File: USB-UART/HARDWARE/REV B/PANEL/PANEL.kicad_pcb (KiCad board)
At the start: 2 copper layers, 81.8 x 90.9 mm, 393 parts, among them P1 USB_OTG, P2 LEFT, P3 RIGHT, U1 FT230XQ-R, U2 AP1117

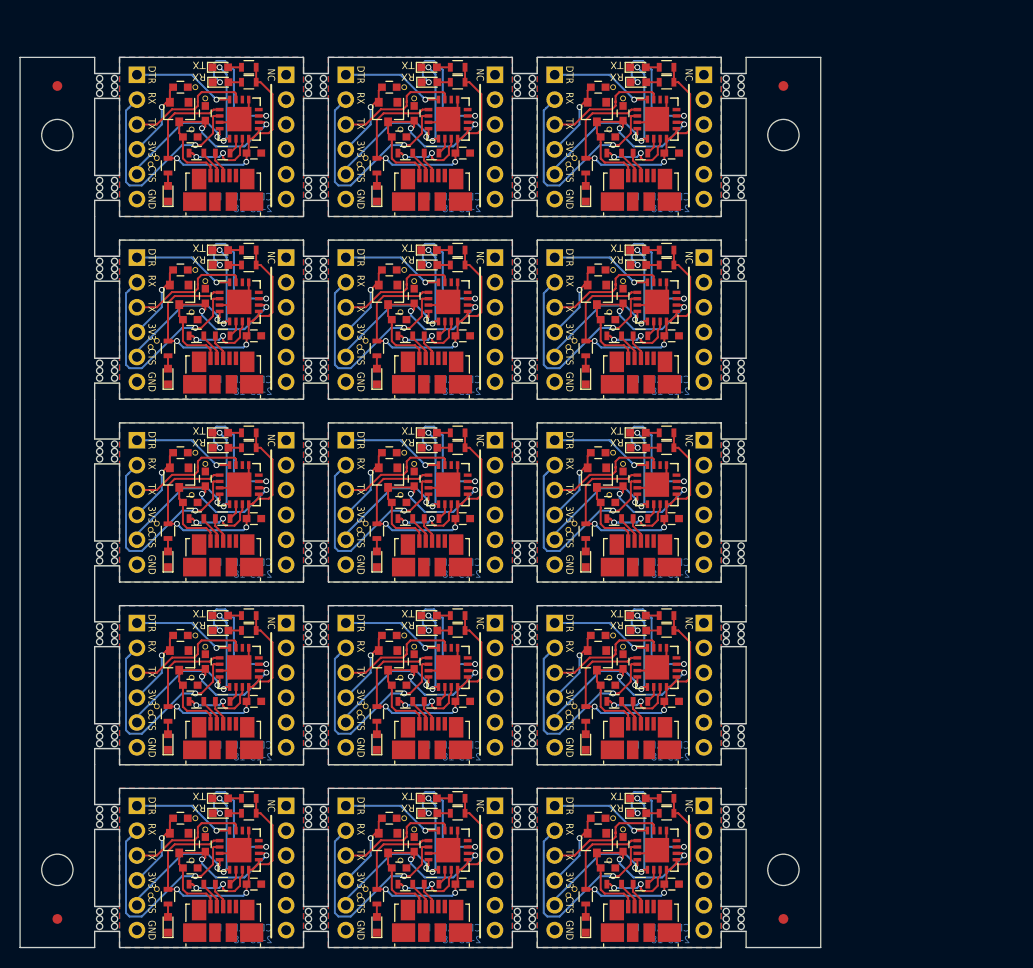
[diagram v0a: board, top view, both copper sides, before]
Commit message: file recovery and updates
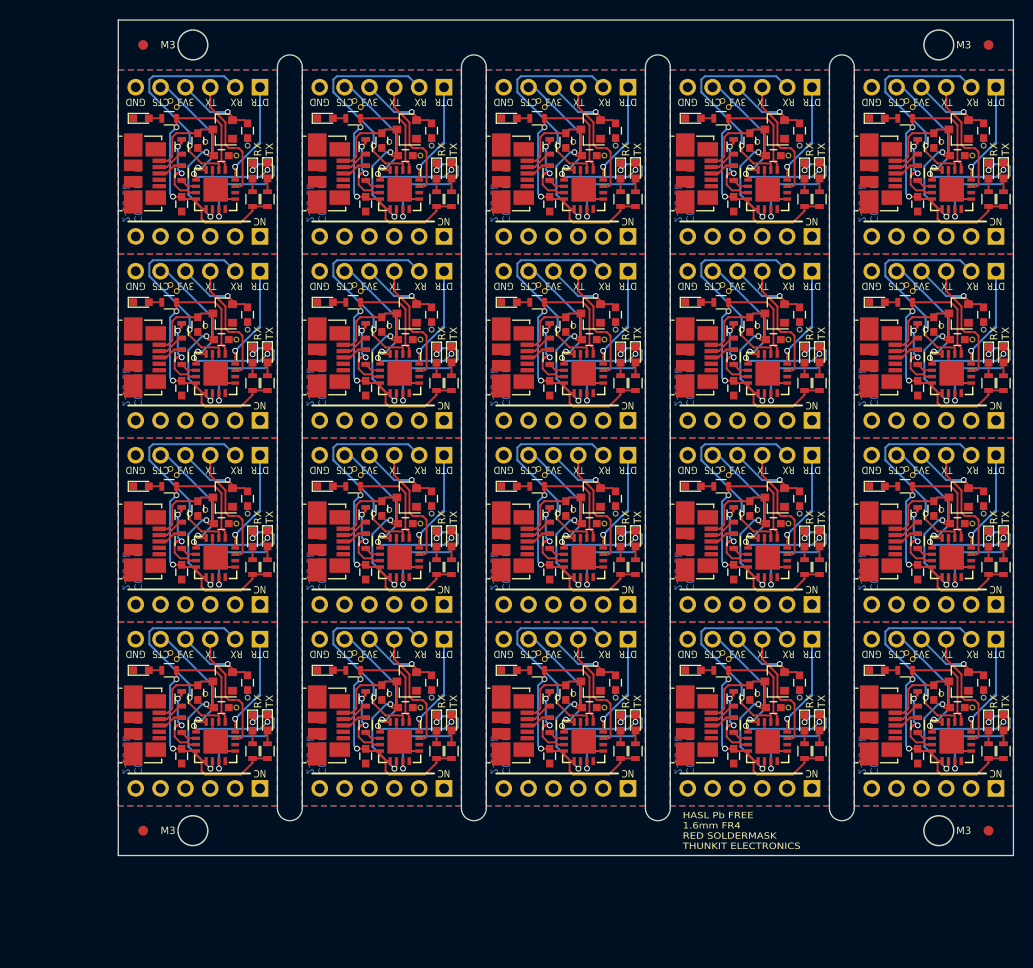
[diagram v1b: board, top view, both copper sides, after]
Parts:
- removed the ? at (164.0, 134.4)
- removed the ? at (121.3, 134.4)
- removed the ? at (125.2, 127.1)
- removed the ? at (126.2, 128.3)
- removed the ? at (124.8, 131.4)
- removed the ? at (146.2, 131.4)
- removed the ? at (146.6, 127.1)
- removed the ? at (125.2, 108.5)
- removed the ? at (124.8, 112.8)
- removed the ? at (121.3, 115.7)
- removed the ? at (120.7, 116.3)
- removed the ? at (163.3, 135.0)
- removed the ? at (126.2, 109.6)
- removed the ? at (164.0, 115.7)
- removed the ? at (163.3, 116.3)
- removed the ? at (167.5, 112.8)
- removed the ? at (167.9, 108.5)
- removed the ? at (168.9, 109.6)
- removed the ? at (146.6, 108.5)
- removed the ? at (142.0, 116.3)
- removed the ? at (142.6, 115.7)
- removed the ? at (146.2, 112.8)
- removed the ? at (167.9, 127.1)
- removed the ? at (147.6, 109.6)
- removed the ? at (168.9, 90.9)
- removed the ? at (167.9, 89.8)
- removed the ? at (167.5, 94.1)
- removed the ? at (164.0, 97.0)
- removed the ? at (163.3, 97.7)
- removed the ? at (147.6, 90.9)
- removed the ? at (146.6, 89.8)
- removed the ? at (146.2, 94.1)
- removed the ? at (124.8, 94.1)
- removed the ? at (167.5, 131.4)
- removed the ? at (120.7, 97.7)
- removed the ? at (121.3, 97.0)
- removed the ? at (126.2, 90.9)
- removed the ? at (125.2, 89.8)
- removed the ? at (142.0, 97.7)
- removed the ? at (142.6, 97.0)
- removed the ? at (167.9, 71.1)
- removed the ? at (168.9, 72.3)
- removed the ? at (164.0, 78.4)
- removed the ? at (163.3, 79.0)
- removed the ? at (142.0, 135.0)
- removed the ? at (167.5, 75.4)
- removed the ? at (147.6, 72.3)
- removed the ? at (124.8, 75.4)
- removed the ? at (125.2, 71.1)
- removed the ? at (126.2, 72.3)
- removed the ? at (142.6, 78.4)
- removed the ? at (146.6, 71.1)
- removed the ? at (146.2, 75.4)
- removed the ? at (121.3, 78.4)
- removed the ? at (120.7, 79.0)
- removed the ? at (142.6, 134.4)
- removed the ? at (142.0, 79.0)
- removed the ? at (167.5, 56.8)
- removed the ? at (163.3, 60.3)
- removed the ? at (164.0, 59.7)
- removed the ? at (168.9, 53.6)
- removed the ? at (167.9, 52.5)
- removed the ? at (146.6, 52.5)
- removed the ? at (142.6, 59.7)
- removed the ? at (142.0, 60.3)
- removed the ? at (146.2, 56.8)
- removed the ? at (147.6, 128.3)
- removed the ? at (147.6, 53.6)
- removed the ? at (168.9, 128.3)
- removed the ? at (120.7, 135.0)
- removed the C1 at (152.5, 135.1)
- removed the C1 at (173.9, 79.1)
- removed the C1 at (131.2, 79.1)
- removed the C1 at (152.5, 79.1)
- removed the C1 at (173.9, 60.5)
- removed the C1 at (152.5, 60.5)
- removed the C1 at (173.9, 135.1)
- removed the C1 at (131.2, 135.1)
- removed the C1 at (131.2, 116.5)
- removed the C1 at (173.9, 116.5)
- removed the C1 at (152.5, 116.5)
- removed the C1 at (173.9, 97.8)
- removed the C1 at (152.5, 97.8)
- removed the C1 at (131.2, 97.8)
- removed the C2 at (147.6, 131.1)
- removed the C2 at (168.9, 75.1)
- removed the C2 at (147.6, 75.1)
- removed the C2 at (126.2, 75.1)
- removed the C2 at (168.9, 56.4)
- removed the C2 at (147.6, 56.4)
- removed the C2 at (168.9, 131.1)
- removed the C2 at (126.2, 131.1)
- removed the C2 at (126.2, 112.4)
- removed the C2 at (168.9, 112.4)
- removed the C2 at (147.6, 112.4)
- removed the C2 at (168.9, 93.7)
- removed the C2 at (147.6, 93.7)
- removed the C2 at (126.2, 93.7)
- removed the C3 at (146.0, 133.5)
- removed the C3 at (167.4, 77.5)
- removed the C3 at (124.7, 77.5)
- removed the C3 at (146.0, 77.5)
- removed the C3 at (167.4, 58.8)
- removed the C3 at (146.0, 58.8)
- removed the C3 at (167.4, 133.5)
- removed the C3 at (124.7, 133.5)
- removed the C3 at (124.7, 114.8)
- removed the C3 at (167.4, 114.8)
- removed the C3 at (146.0, 114.8)
- removed the C3 at (167.4, 96.1)
- removed the C3 at (124.7, 96.1)
- removed the C3 at (146.0, 96.1)
- removed the C4 at (166.4, 128.4)
- removed the C4 at (166.4, 72.4)
- removed the C4 at (123.7, 72.4)
- removed the C4 at (145.0, 72.4)
- removed the C4 at (166.4, 53.7)
- removed the C4 at (145.0, 53.7)
- removed the C4 at (123.7, 128.4)
- removed the C4 at (145.0, 128.4)
- removed the C4 at (123.7, 109.7)
- removed the C4 at (166.4, 109.7)
- removed the C4 at (145.0, 109.7)
- removed the C4 at (166.4, 91.1)
- removed the C4 at (145.0, 91.1)
- removed the C4 at (123.7, 91.1)
- removed the D1 at (165.1, 139.3)
- removed the D1 at (165.1, 83.3)
- removed the D1 at (122.4, 83.3)
- removed the D1 at (143.8, 83.3)
- removed the D1 at (165.1, 64.6)
- removed the D1 at (143.8, 64.6)
- removed the D1 at (143.8, 139.3)
- removed the D1 at (122.4, 139.3)
- removed the D1 at (122.4, 120.6)
- removed the D1 at (165.1, 120.6)
- removed the D1 at (143.8, 120.6)
- removed the D1 at (165.1, 101.9)
- removed the D1 at (122.4, 101.9)
- removed the D1 at (143.8, 101.9)
- removed the D2 at (149.1, 126.4)
- removed the D2 at (170.4, 70.4)
- removed the D2 at (149.1, 70.4)
- removed the D2 at (127.8, 70.4)
- removed the D2 at (170.4, 51.7)
- removed the D2 at (149.1, 51.7)
- removed the D2 at (170.4, 126.4)
- removed the D2 at (127.8, 126.4)
- removed the D2 at (127.8, 107.7)
- removed the D2 at (170.4, 107.7)
- removed the D2 at (149.1, 107.7)
- removed the D2 at (170.4, 89.0)
- removed the D2 at (149.1, 89.0)
- removed the D2 at (127.8, 89.0)
- removed the D3 at (149.1, 127.9)
- removed the D3 at (170.5, 71.9)
- removed the D3 at (149.1, 71.9)
- removed the D3 at (127.8, 71.9)
- removed the D3 at (170.5, 53.2)
- removed the D3 at (149.1, 53.2)
- removed the D3 at (170.5, 127.9)
- removed the D3 at (127.8, 127.9)
- removed the D3 at (127.8, 109.2)
- removed the D3 at (170.5, 109.2)
- removed the D3 at (149.1, 109.2)
- removed the D3 at (170.5, 90.6)
- removed the D3 at (149.1, 90.6)
- removed the D3 at (127.8, 90.6)
- removed the G*** at (144.1, 138.0)
- removed the G*** at (144.1, 82.0)
- removed the G*** at (122.8, 82.0)
- removed the G*** at (165.5, 82.0)
- removed the G*** at (165.5, 63.4)
- removed the G*** at (144.1, 63.4)
- removed the G*** at (122.8, 138.0)
- removed the G*** at (165.5, 138.0)
- removed the G*** at (165.5, 119.4)
- removed the G*** at (144.1, 119.4)
- removed the G*** at (122.8, 119.4)
- removed the G*** at (122.8, 100.7)
- removed the G*** at (144.1, 100.7)
- removed the G*** at (165.5, 100.7)
- removed the P1 at (149.4, 140.1)
- removed the P1 at (170.7, 84.1)
- removed the P1 at (128.1, 84.1)
- removed the P1 at (149.4, 84.1)
- removed the P1 at (170.7, 65.4)
- removed the P1 at (149.4, 65.4)
- removed the P1 at (170.7, 140.1)
- removed the P1 at (128.1, 140.1)
- removed the P1 at (128.1, 121.4)
- removed the P1 at (170.7, 121.4)
- removed the P1 at (149.4, 121.4)
- removed the P1 at (170.7, 102.7)
- removed the P1 at (149.4, 102.7)
- removed the P1 at (128.1, 102.7)
- removed the P2 at (140.6, 127.1)
- removed the P2 at (140.6, 71.1)
- removed the P2 at (119.3, 71.1)
- removed the P2 at (161.9, 71.1)
- removed the P2 at (161.9, 52.5)
- removed the P2 at (140.6, 52.5)
- removed the P2 at (119.3, 127.1)
- removed the P2 at (161.9, 127.1)
- removed the P2 at (161.9, 108.5)
- removed the P2 at (140.6, 108.5)
- removed the P2 at (119.3, 108.5)
- removed the P2 at (140.6, 89.8)
- removed the P2 at (119.3, 89.8)
- removed the P2 at (161.9, 89.8)
- removed the P3 at (134.5, 127.1)
- removed the P3 at (134.5, 71.1)
- removed the P3 at (155.8, 71.1)
- removed the P3 at (177.2, 71.1)
- removed the P3 at (177.2, 52.5)
- removed the P3 at (155.8, 52.5)
- removed the P3 at (155.8, 127.1)
- removed the P3 at (177.2, 127.1)
- removed the P3 at (155.8, 108.5)
- removed the P3 at (177.2, 108.5)
- removed the P3 at (134.5, 108.5)
- removed the P3 at (134.5, 89.8)
- removed the P3 at (155.8, 89.8)
- removed the P3 at (177.2, 89.8)
- removed the R1 at (146.7, 135.1)
- removed the R1 at (168.0, 79.1)
- removed the R1 at (125.3, 79.1)
- removed the R1 at (146.7, 79.1)
- removed the R1 at (168.0, 60.5)
- removed the R1 at (146.7, 60.5)
- removed the R1 at (168.0, 135.1)
- removed the R1 at (125.3, 135.1)
- removed the R1 at (125.3, 116.5)
- removed the R1 at (168.0, 116.5)
- removed the R1 at (146.7, 116.5)
- removed the R1 at (168.0, 97.8)
- removed the R1 at (146.7, 97.8)
- removed the R1 at (125.3, 97.8)
- removed the R2 at (149.4, 135.1)
- removed the R2 at (170.7, 79.1)
- removed the R2 at (128.0, 79.1)
- removed the R2 at (149.4, 79.1)
- removed the R2 at (170.7, 60.5)
- removed the R2 at (149.4, 60.5)
- removed the R2 at (170.7, 135.1)
- removed the R2 at (128.0, 135.1)
- removed the R2 at (128.0, 116.5)
- removed the R2 at (170.7, 116.5)
- removed the R2 at (149.4, 116.5)
- removed the R2 at (170.7, 97.8)
- removed the R2 at (149.4, 97.8)
- removed the R2 at (128.0, 97.8)
- removed the R3 at (165.1, 136.4)
- removed the R3 at (165.1, 80.4)
- removed the R3 at (122.4, 80.4)
- removed the R3 at (143.8, 80.4)
- removed the R3 at (165.1, 61.7)
- removed the R3 at (143.8, 61.7)
- removed the R3 at (143.8, 136.4)
- removed the R3 at (122.4, 136.4)
- removed the R3 at (122.4, 117.7)
- removed the R3 at (165.1, 117.7)
- removed the R3 at (143.8, 117.7)
- removed the R3 at (165.1, 99.1)
- removed the R3 at (122.4, 99.1)
- removed the R3 at (143.8, 99.1)
- removed the R4 at (152.0, 126.4)
- removed the R4 at (173.4, 70.4)
- removed the R4 at (152.0, 70.4)
- removed the R4 at (130.7, 70.4)
- removed the R4 at (173.4, 51.7)
- removed the R4 at (152.0, 51.7)
- removed the R4 at (173.4, 126.4)
- removed the R4 at (130.7, 126.4)
- removed the R4 at (130.7, 107.7)
- removed the R4 at (173.4, 107.7)
- removed the R4 at (152.0, 107.7)
- removed the R4 at (173.4, 89.0)
- removed the R4 at (152.0, 89.0)
- removed the R4 at (130.7, 89.0)
- removed the R5 at (152.0, 127.9)
- removed the R5 at (173.4, 71.9)
- removed the R5 at (152.0, 71.9)
- removed the R5 at (130.7, 71.9)
- removed the R5 at (173.4, 53.2)
- removed the R5 at (152.0, 53.2)
- removed the R5 at (173.4, 127.9)
- removed the R5 at (130.7, 127.9)
- removed the R5 at (130.7, 109.2)
- removed the R5 at (173.4, 109.2)
- removed the R5 at (152.0, 109.2)
- removed the R5 at (173.4, 90.6)
- removed the R5 at (152.0, 90.6)
- removed the R5 at (130.7, 90.6)
- removed the REF** at (185.3, 53.6)
- removed the REF** at (180.2, 138.7)
- removed the REF** at (180.2, 128.3)
- removed the REF** at (116.2, 128.3)
- removed the REF** at (116.2, 138.7)
- removed the REF** at (137.5, 128.3)
- removed the REF** at (116.2, 120.0)
- removed the REF** at (116.2, 109.6)
- removed the REF** at (180.2, 120.0)
- removed the REF** at (158.9, 120.0)
- removed the REF** at (158.9, 109.6)
- removed the REF** at (185.3, 58.6)
- removed the REF** at (180.2, 109.6)
- removed the REF** at (137.5, 120.0)
- removed the REF** at (137.5, 109.6)
- removed the REF** at (180.2, 101.3)
- removed the REF** at (180.2, 90.9)
- removed the REF** at (158.9, 101.3)
- removed the REF** at (158.9, 90.9)
- removed the REF** at (137.5, 90.9)
- removed the REF** at (116.2, 90.9)
- removed the REF** at (116.2, 101.3)
- removed the REF** at (185.3, 133.7)
- removed the REF** at (137.5, 101.3)
- removed the REF** at (180.2, 72.3)
- removed the REF** at (158.9, 82.7)
- removed the REF** at (180.2, 82.7)
- removed the REF** at (158.9, 72.3)
- removed the REF** at (116.2, 72.3)
- removed the REF** at (137.5, 82.7)
- removed the REF** at (137.5, 72.3)
- removed the REF** at (116.2, 82.7)
- removed the REF** at (180.2, 53.6)
- removed the REF** at (185.3, 138.7)
- removed the REF** at (180.2, 64.0)
- removed the REF** at (158.9, 53.6)
- removed the REF** at (158.9, 64.0)
- removed the REF** at (137.5, 64.0)
- removed the REF** at (137.5, 53.6)
- removed the REF** at (116.2, 64.0)
- removed the REF** at (116.2, 53.6)
- removed the REF** at (111.1, 133.7)
- removed the REF** at (111.1, 138.7)
- removed the REF** at (111.1, 58.6)
- removed the REF** at (111.1, 53.6)
- removed the REF** at (158.9, 138.7)
- removed the REF** at (158.9, 128.3)
- removed the REF** at (137.5, 138.7)
- removed the U1 at (151.0, 131.7)
- removed the U1 at (172.4, 75.7)
- removed the U1 at (129.7, 75.7)
- removed the U1 at (151.0, 75.7)
- removed the U1 at (172.4, 57.0)
- removed the U1 at (151.0, 57.0)
- removed the U1 at (172.4, 131.7)
- removed the U1 at (129.7, 131.7)
- removed the U1 at (129.7, 113.0)
- removed the U1 at (172.4, 113.0)
- removed the U1 at (151.0, 113.0)
- removed the U1 at (172.4, 94.3)
- removed the U1 at (151.0, 94.3)
- removed the U1 at (129.7, 94.3)
- removed the U2 at (166.2, 130.9)
- removed the U2 at (166.2, 74.9)
- removed the U2 at (123.6, 74.9)
- removed the U2 at (144.9, 74.9)
- removed the U2 at (166.2, 56.3)
- removed the U2 at (144.9, 56.3)
- removed the U2 at (123.6, 130.9)
- removed the U2 at (144.9, 130.9)
- removed the U2 at (123.6, 112.3)
- removed the U2 at (166.2, 112.3)
- removed the U2 at (144.9, 112.3)
- removed the U2 at (166.2, 93.6)
- removed the U2 at (144.9, 93.6)
- removed the U2 at (123.6, 93.6)
- added ?: , MOD:GND VIA, F.Cu at (202.7, 78.1)
- added ?: , MOD:GND VIA, F.Cu at (205.9, 117.1)
- added ?: , MOD:GND VIA, F.Cu at (207.0, 116.1)
- added ?: , MOD:GND VIA, F.Cu at (199.1, 111.5)
- added ?: , MOD:GND VIA, F.Cu at (199.8, 112.1)
- added ?: , MOD:GND VIA, F.Cu at (199.8, 74.5)
- added ?: , MOD:GND VIA, F.Cu at (199.1, 73.9)
- added ?: , MOD:GND VIA, F.Cu at (202.7, 59.3)
- added ?: , MOD:GND VIA, F.Cu at (205.9, 60.7)
- added ?: , MOD:GND VIA, F.Cu at (199.1, 55.1)
- added ?: , MOD:GND VIA, F.Cu at (199.8, 55.8)
- added ?: , MOD:GND VIA, F.Cu at (207.0, 78.5)
- added ?: , MOD:GND VIA, F.Cu at (207.0, 59.7)
- added ?: , MOD:GND VIA, F.Cu at (183.9, 78.1)
- added ?: , MOD:GND VIA, F.Cu at (188.2, 78.5)
- added ?: , MOD:GND VIA, F.Cu at (187.1, 79.5)
- added ?: , MOD:GND VIA, F.Cu at (180.3, 92.7)
- added ?: , MOD:GND VIA, F.Cu at (181.0, 93.3)
- added ?: , MOD:GND VIA, F.Cu at (188.2, 97.3)
- added ?: , MOD:GND VIA, F.Cu at (183.9, 96.9)
- added ?: , MOD:GND VIA, F.Cu at (187.1, 98.3)
- added ?: , MOD:GND VIA, F.Cu at (183.9, 115.7)
- added ?: , MOD:GND VIA, F.Cu at (205.9, 79.5)
- added ?: , MOD:GND VIA, F.Cu at (187.1, 117.1)
- added ?: , MOD:GND VIA, F.Cu at (188.2, 116.1)
- added ?: , MOD:GND VIA, F.Cu at (180.3, 111.5)
- added ?: , MOD:GND VIA, F.Cu at (181.0, 112.1)
- added ?: , MOD:GND VIA, F.Cu at (181.0, 74.5)
- added ?: , MOD:GND VIA, F.Cu at (180.3, 73.9)
- added ?: , MOD:GND VIA, F.Cu at (183.9, 59.3)
- added ?: , MOD:GND VIA, F.Cu at (187.1, 60.7)
- added ?: , MOD:GND VIA, F.Cu at (180.3, 55.1)
- added ?: , MOD:GND VIA, F.Cu at (181.0, 55.8)
- added ?: , MOD:GND VIA, F.Cu at (199.1, 92.7)
- added ?: , MOD:GND VIA, F.Cu at (188.2, 59.7)
- added ?: , MOD:GND VIA, F.Cu at (165.1, 78.1)
- added ?: , MOD:GND VIA, F.Cu at (169.4, 78.5)
- added ?: , MOD:GND VIA, F.Cu at (168.3, 79.5)
- added ?: , MOD:GND VIA, F.Cu at (161.5, 92.7)
- added ?: , MOD:GND VIA, F.Cu at (162.2, 93.3)
- added ?: , MOD:GND VIA, F.Cu at (169.4, 97.3)
- added ?: , MOD:GND VIA, F.Cu at (165.1, 96.9)
- added ?: , MOD:GND VIA, F.Cu at (168.3, 98.3)
- added ?: , MOD:GND VIA, F.Cu at (165.1, 115.7)
- added ?: , MOD:GND VIA, F.Cu at (199.8, 93.3)
- added ?: , MOD:GND VIA, F.Cu at (168.3, 117.1)
- added ?: , MOD:GND VIA, F.Cu at (169.4, 116.1)
- added ?: , MOD:GND VIA, F.Cu at (161.5, 111.5)
- added ?: , MOD:GND VIA, F.Cu at (162.2, 112.1)
- added ?: , MOD:GND VIA, F.Cu at (162.2, 74.5)
- added ?: , MOD:GND VIA, F.Cu at (161.5, 73.9)
- added ?: , MOD:GND VIA, F.Cu at (165.1, 59.3)
- added ?: , MOD:GND VIA, F.Cu at (168.3, 60.7)
- added ?: , MOD:GND VIA, F.Cu at (161.5, 55.1)
- added ?: , MOD:GND VIA, F.Cu at (162.2, 55.8)
- added ?: , MOD:GND VIA, F.Cu at (207.0, 97.3)
- added ?: , MOD:GND VIA, F.Cu at (169.4, 59.7)
- added ?: , MOD:GND VIA, F.Cu at (146.3, 78.1)
- added ?: , MOD:GND VIA, F.Cu at (150.6, 78.5)
- added ?: , MOD:GND VIA, F.Cu at (149.5, 79.5)
- added ?: , MOD:GND VIA, F.Cu at (142.7, 92.7)
- added ?: , MOD:GND VIA, F.Cu at (143.4, 93.3)
- added ?: , MOD:GND VIA, F.Cu at (150.6, 97.3)
- added ?: , MOD:GND VIA, F.Cu at (146.3, 96.9)
- added ?: , MOD:GND VIA, F.Cu at (149.5, 98.3)
- added ?: , MOD:GND VIA, F.Cu at (146.3, 115.7)
- added ?: , MOD:GND VIA, F.Cu at (202.7, 96.9)
- added ?: , MOD:GND VIA, F.Cu at (149.5, 117.1)
- added ?: , MOD:GND VIA, F.Cu at (150.6, 116.1)
- added ?: , MOD:GND VIA, F.Cu at (142.7, 111.5)
- added ?: , MOD:GND VIA, F.Cu at (143.4, 112.1)
- added ?: , MOD:GND VIA, F.Cu at (143.4, 74.5)
- added ?: , MOD:GND VIA, F.Cu at (142.7, 73.9)
- added ?: , MOD:GND VIA, F.Cu at (146.3, 59.3)
- added ?: , MOD:GND VIA, F.Cu at (149.5, 60.7)
- added ?: , MOD:GND VIA, F.Cu at (142.7, 55.1)
- added ?: , MOD:GND VIA, F.Cu at (143.4, 55.8)
- added ?: , MOD:GND VIA, F.Cu at (205.9, 98.3)
- added ?: , MOD:GND VIA, F.Cu at (150.6, 59.7)
- added ?: , MOD:GND VIA, F.Cu at (124.0, 111.5)
- added ?: , MOD:GND VIA, F.Cu at (124.6, 112.1)
- added ?: , MOD:GND VIA, F.Cu at (127.5, 115.7)
- added ?: , MOD:GND VIA, F.Cu at (131.8, 116.1)
- added ?: , MOD:GND VIA, F.Cu at (130.7, 117.1)
- added ?: , MOD:GND VIA, F.Cu at (130.7, 98.3)
- added ?: , MOD:GND VIA, F.Cu at (131.8, 97.3)
- added ?: , MOD:GND VIA, F.Cu at (127.5, 96.9)
- added ?: , MOD:GND VIA, F.Cu at (124.6, 93.3)
- added ?: , MOD:GND VIA, F.Cu at (202.7, 115.7)
- added ?: , MOD:GND VIA, F.Cu at (124.0, 92.7)
- added ?: , MOD:GND VIA, F.Cu at (127.5, 78.1)
- added ?: , MOD:GND VIA, F.Cu at (130.7, 79.5)
- added ?: , MOD:GND VIA, F.Cu at (131.8, 78.5)
- added ?: , MOD:GND VIA, F.Cu at (124.0, 73.9)
- added ?: , MOD:GND VIA, F.Cu at (124.6, 74.5)
- added C1: 1uF, Capacitors_SMD:C_0603, F.Cu at (199.0, 84.5)
- added C1: 1uF, Capacitors_SMD:C_0603, F.Cu at (161.4, 103.3)
- added C1: 1uF, Capacitors_SMD:C_0603, F.Cu at (161.4, 122.1)
- added C1: 1uF, Capacitors_SMD:C_0603, F.Cu at (161.4, 65.7)
- added C1: 1uF, Capacitors_SMD:C_0603, F.Cu at (142.6, 84.5)
- added C1: 1uF, Capacitors_SMD:C_0603, F.Cu at (142.6, 103.3)
- added C1: 1uF, Capacitors_SMD:C_0603, F.Cu at (142.6, 122.1)
- added C1: 1uF, Capacitors_SMD:C_0603, F.Cu at (142.6, 65.7)
- added C1: 1uF, Capacitors_SMD:C_0603, F.Cu at (123.8, 122.1)
- added C1: 1uF, Capacitors_SMD:C_0603, F.Cu at (123.8, 103.3)
- added C1: 1uF, Capacitors_SMD:C_0603, F.Cu at (123.8, 84.5)
- added C1: 1uF, Capacitors_SMD:C_0603, F.Cu at (199.0, 103.3)
- added C1: 1uF, Capacitors_SMD:C_0603, F.Cu at (199.0, 122.1)
- added C1: 1uF, Capacitors_SMD:C_0603, F.Cu at (199.0, 65.7)
- added C1: 1uF, Capacitors_SMD:C_0603, F.Cu at (180.2, 84.5)
- added C1: 1uF, Capacitors_SMD:C_0603, F.Cu at (180.2, 103.3)
- added C1: 1uF, Capacitors_SMD:C_0603, F.Cu at (180.2, 122.1)
- added C1: 1uF, Capacitors_SMD:C_0603, F.Cu at (180.2, 65.7)
- added C1: 1uF, Capacitors_SMD:C_0603, F.Cu at (161.4, 84.5)
- added C2: 1uF, Capacitors_SMD:C_0603, F.Cu at (203.1, 79.5)
- added C2: 1uF, Capacitors_SMD:C_0603, F.Cu at (165.5, 98.3)
- added C2: 1uF, Capacitors_SMD:C_0603, F.Cu at (165.5, 117.1)
- added C2: 1uF, Capacitors_SMD:C_0603, F.Cu at (165.5, 60.7)
- added C2: 1uF, Capacitors_SMD:C_0603, F.Cu at (146.7, 79.5)
- added C2: 1uF, Capacitors_SMD:C_0603, F.Cu at (146.7, 98.3)
- added C2: 1uF, Capacitors_SMD:C_0603, F.Cu at (146.7, 117.1)
- added C2: 1uF, Capacitors_SMD:C_0603, F.Cu at (146.7, 60.7)
- added C2: 1uF, Capacitors_SMD:C_0603, F.Cu at (127.9, 117.1)
- added C2: 1uF, Capacitors_SMD:C_0603, F.Cu at (127.9, 98.3)
- added C2: 1uF, Capacitors_SMD:C_0603, F.Cu at (127.9, 79.5)
- added C2: 1uF, Capacitors_SMD:C_0603, F.Cu at (203.1, 98.3)
- added C2: 1uF, Capacitors_SMD:C_0603, F.Cu at (203.1, 117.1)
- added C2: 1uF, Capacitors_SMD:C_0603, F.Cu at (203.1, 60.7)
- added C2: 1uF, Capacitors_SMD:C_0603, F.Cu at (184.3, 79.5)
- added C2: 1uF, Capacitors_SMD:C_0603, F.Cu at (184.3, 98.3)
- added C2: 1uF, Capacitors_SMD:C_0603, F.Cu at (184.3, 117.1)
- added C2: 1uF, Capacitors_SMD:C_0603, F.Cu at (184.3, 60.7)
- added C2: 1uF, Capacitors_SMD:C_0603, F.Cu at (165.5, 79.5)
- added C3: 1uF, Capacitors_SMD:C_0603, F.Cu at (200.7, 78.0)
- added C3: 1uF, Capacitors_SMD:C_0603, F.Cu at (163.1, 96.8)
- added C3: 1uF, Capacitors_SMD:C_0603, F.Cu at (163.1, 115.6)
- added C3: 1uF, Capacitors_SMD:C_0603, F.Cu at (163.1, 59.2)
- added C3: 1uF, Capacitors_SMD:C_0603, F.Cu at (144.3, 78.0)
- added C3: 1uF, Capacitors_SMD:C_0603, F.Cu at (144.3, 96.8)
- added C3: 1uF, Capacitors_SMD:C_0603, F.Cu at (144.3, 115.6)
- added C3: 1uF, Capacitors_SMD:C_0603, F.Cu at (144.3, 59.2)
- added C3: 1uF, Capacitors_SMD:C_0603, F.Cu at (125.5, 115.6)
- added C3: 1uF, Capacitors_SMD:C_0603, F.Cu at (125.5, 96.8)
- added C3: 1uF, Capacitors_SMD:C_0603, F.Cu at (125.5, 78.0)
- added C3: 1uF, Capacitors_SMD:C_0603, F.Cu at (200.7, 96.8)
- added C3: 1uF, Capacitors_SMD:C_0603, F.Cu at (200.7, 115.6)
- added C3: 1uF, Capacitors_SMD:C_0603, F.Cu at (200.7, 59.2)
- added C3: 1uF, Capacitors_SMD:C_0603, F.Cu at (181.9, 78.0)
- added C3: 1uF, Capacitors_SMD:C_0603, F.Cu at (181.9, 96.8)
- added C3: 1uF, Capacitors_SMD:C_0603, F.Cu at (181.9, 115.6)
- added C3: 1uF, Capacitors_SMD:C_0603, F.Cu at (181.9, 59.2)
- added C3: 1uF, Capacitors_SMD:C_0603, F.Cu at (163.1, 78.0)
- added C4: 1uF, Capacitors_SMD:C_0603, F.Cu at (205.7, 77.0)
- added C4: 1uF, Capacitors_SMD:C_0603, F.Cu at (168.1, 95.8)
- added C4: 1uF, Capacitors_SMD:C_0603, F.Cu at (168.1, 114.6)
- added C4: 1uF, Capacitors_SMD:C_0603, F.Cu at (168.1, 58.2)
- added C4: 1uF, Capacitors_SMD:C_0603, F.Cu at (149.4, 77.0)
- added C4: 1uF, Capacitors_SMD:C_0603, F.Cu at (149.4, 95.8)
- added C4: 1uF, Capacitors_SMD:C_0603, F.Cu at (149.4, 114.6)
- added C4: 1uF, Capacitors_SMD:C_0603, F.Cu at (149.4, 58.2)
- added C4: 1uF, Capacitors_SMD:C_0603, F.Cu at (130.6, 114.6)
- added C4: 1uF, Capacitors_SMD:C_0603, F.Cu at (130.6, 95.8)
- added C4: 1uF, Capacitors_SMD:C_0603, F.Cu at (130.6, 77.0)
- added C4: 1uF, Capacitors_SMD:C_0603, F.Cu at (205.7, 95.8)
- added C4: 1uF, Capacitors_SMD:C_0603, F.Cu at (205.7, 114.6)
- added C4: 1uF, Capacitors_SMD:C_0603, F.Cu at (205.7, 58.2)
- added C4: 1uF, Capacitors_SMD:C_0603, F.Cu at (186.9, 77.0)
- added C4: 1uF, Capacitors_SMD:C_0603, F.Cu at (186.9, 95.8)
- added C4: 1uF, Capacitors_SMD:C_0603, F.Cu at (186.9, 114.6)
- added C4: 1uF, Capacitors_SMD:C_0603, F.Cu at (186.9, 58.2)
- added C4: 1uF, Capacitors_SMD:C_0603, F.Cu at (168.1, 77.0)
- added D1: LED, LEDs:LED_0603, F.Cu at (194.9, 94.5)
- added D1: LED, LEDs:LED_0603, F.Cu at (157.3, 113.3)
- added D1: LED, LEDs:LED_0603, F.Cu at (157.3, 75.7)
- added D1: LED, LEDs:LED_0603, F.Cu at (157.3, 56.9)
- added D1: LED, LEDs:LED_0603, F.Cu at (138.5, 94.5)
- added D1: LED, LEDs:LED_0603, F.Cu at (138.5, 113.3)
- added D1: LED, LEDs:LED_0603, F.Cu at (138.5, 75.7)
- added D1: LED, LEDs:LED_0603, F.Cu at (138.5, 56.9)
- added D1: LED, LEDs:LED_0603, F.Cu at (119.7, 113.3)
- added D1: LED, LEDs:LED_0603, F.Cu at (119.7, 94.5)
- added D1: LED, LEDs:LED_0603, F.Cu at (119.7, 75.7)
- added D1: LED, LEDs:LED_0603, F.Cu at (194.9, 113.3)
- added D1: LED, LEDs:LED_0603, F.Cu at (194.9, 75.7)
- added D1: LED, LEDs:LED_0603, F.Cu at (194.9, 56.9)
- added D1: LED, LEDs:LED_0603, F.Cu at (176.1, 94.5)
- added D1: LED, LEDs:LED_0603, F.Cu at (176.1, 113.3)
- added D1: LED, LEDs:LED_0603, F.Cu at (176.1, 75.7)
- added D1: LED, LEDs:LED_0603, F.Cu at (176.1, 56.9)
- added D1: LED, LEDs:LED_0603, F.Cu at (157.3, 94.5)
- added D2: TX, LEDs:LED_0603, F.Cu at (207.8, 81.0)
- added D2: TX, LEDs:LED_0603, F.Cu at (170.2, 99.8)
- added D2: TX, LEDs:LED_0603, F.Cu at (170.2, 118.6)
- added D2: TX, LEDs:LED_0603, F.Cu at (170.2, 62.2)
- added D2: TX, LEDs:LED_0603, F.Cu at (151.4, 81.0)
- added D2: TX, LEDs:LED_0603, F.Cu at (151.4, 99.8)
- added D2: TX, LEDs:LED_0603, F.Cu at (151.4, 118.6)
- added D2: TX, LEDs:LED_0603, F.Cu at (151.4, 62.2)
- added D2: TX, LEDs:LED_0603, F.Cu at (132.6, 118.6)
- added D2: TX, LEDs:LED_0603, F.Cu at (132.6, 99.8)
- added D2: TX, LEDs:LED_0603, F.Cu at (132.6, 81.0)
- added D2: TX, LEDs:LED_0603, F.Cu at (207.8, 99.8)
- added D2: TX, LEDs:LED_0603, F.Cu at (207.8, 118.6)
- added D2: TX, LEDs:LED_0603, F.Cu at (207.8, 62.2)
- added D2: TX, LEDs:LED_0603, F.Cu at (189.0, 81.0)
- added D2: TX, LEDs:LED_0603, F.Cu at (189.0, 99.8)
- added D2: TX, LEDs:LED_0603, F.Cu at (189.0, 118.6)
- added D2: TX, LEDs:LED_0603, F.Cu at (189.0, 62.2)
- added D2: TX, LEDs:LED_0603, F.Cu at (170.2, 81.0)
- added D3: RX, LEDs:LED_0603, F.Cu at (206.2, 81.1)
- added D3: RX, LEDs:LED_0603, F.Cu at (168.7, 99.9)
- added D3: RX, LEDs:LED_0603, F.Cu at (168.7, 118.7)
- added D3: RX, LEDs:LED_0603, F.Cu at (168.7, 62.3)
- added D3: RX, LEDs:LED_0603, F.Cu at (149.9, 81.1)
- added D3: RX, LEDs:LED_0603, F.Cu at (149.9, 99.9)
- added D3: RX, LEDs:LED_0603, F.Cu at (149.9, 118.7)
- added D3: RX, LEDs:LED_0603, F.Cu at (149.9, 62.3)
- added D3: RX, LEDs:LED_0603, F.Cu at (131.1, 118.7)
- added D3: RX, LEDs:LED_0603, F.Cu at (131.1, 99.9)
- added D3: RX, LEDs:LED_0603, F.Cu at (131.1, 81.1)
- added D3: RX, LEDs:LED_0603, F.Cu at (206.2, 99.9)
- added D3: RX, LEDs:LED_0603, F.Cu at (206.2, 118.7)
- added D3: RX, LEDs:LED_0603, F.Cu at (206.2, 62.3)
- added D3: RX, LEDs:LED_0603, F.Cu at (187.5, 81.1)
- added D3: RX, LEDs:LED_0603, F.Cu at (187.5, 99.9)
- added D3: RX, LEDs:LED_0603, F.Cu at (187.5, 118.7)
- added D3: RX, LEDs:LED_0603, F.Cu at (187.5, 62.3)
- added D3: RX, LEDs:LED_0603, F.Cu at (168.7, 81.1)
- added G***: LOGO, MOD:lightning, B.Cu at (196.1, 113.7)
- added G***: LOGO, MOD:lightning, B.Cu at (158.5, 94.9)
- added G***: LOGO, MOD:lightning, B.Cu at (158.5, 57.3)
- added G***: LOGO, MOD:lightning, B.Cu at (158.5, 76.1)
- added G***: LOGO, MOD:lightning, B.Cu at (139.7, 113.7)
- added G***: LOGO, MOD:lightning, B.Cu at (139.7, 94.9)
- added G***: LOGO, MOD:lightning, B.Cu at (139.7, 57.3)
- added G***: LOGO, MOD:lightning, B.Cu at (139.7, 76.1)
- added G***: LOGO, MOD:lightning, B.Cu at (120.9, 113.7)
- added G***: LOGO, MOD:lightning, B.Cu at (120.9, 94.9)
- added G***: LOGO, MOD:lightning, B.Cu at (120.9, 76.1)
- added G***: LOGO, MOD:lightning, B.Cu at (196.1, 94.9)
- added G***: LOGO, MOD:lightning, B.Cu at (196.1, 57.3)
- added G***: LOGO, MOD:lightning, B.Cu at (196.1, 76.1)
- added G***: LOGO, MOD:lightning, B.Cu at (177.3, 113.7)
- added G***: LOGO, MOD:lightning, B.Cu at (177.3, 94.9)
- added G***: LOGO, MOD:lightning, B.Cu at (177.3, 57.3)
- added G***: LOGO, MOD:lightning, B.Cu at (177.3, 76.1)
- added G***: LOGO, MOD:lightning, B.Cu at (158.5, 113.7)
- added P1: USB_OTG, Connectors_USB:USB_Micro-B_Molex_47346-0001, F.Cu at (194.1, 81.3)
- added P1: USB_OTG, Connectors_USB:USB_Micro-B_Molex_47346-0001, F.Cu at (156.5, 100.1)
- added P1: USB_OTG, Connectors_USB:USB_Micro-B_Molex_47346-0001, F.Cu at (156.5, 118.9)
- added P1: USB_OTG, Connectors_USB:USB_Micro-B_Molex_47346-0001, F.Cu at (156.5, 62.5)
- added P1: USB_OTG, Connectors_USB:USB_Micro-B_Molex_47346-0001, F.Cu at (137.7, 81.3)
- added P1: USB_OTG, Connectors_USB:USB_Micro-B_Molex_47346-0001, F.Cu at (137.7, 100.1)
- added P1: USB_OTG, Connectors_USB:USB_Micro-B_Molex_47346-0001, F.Cu at (137.7, 118.9)
- added P1: USB_OTG, Connectors_USB:USB_Micro-B_Molex_47346-0001, F.Cu at (137.7, 62.5)
- added P1: USB_OTG, Connectors_USB:USB_Micro-B_Molex_47346-0001, F.Cu at (118.9, 118.9)
- added P1: USB_OTG, Connectors_USB:USB_Micro-B_Molex_47346-0001, F.Cu at (118.9, 100.1)
- added P1: USB_OTG, Connectors_USB:USB_Micro-B_Molex_47346-0001, F.Cu at (118.9, 81.3)
- added P1: USB_OTG, Connectors_USB:USB_Micro-B_Molex_47346-0001, F.Cu at (194.1, 100.1)
- added P1: USB_OTG, Connectors_USB:USB_Micro-B_Molex_47346-0001, F.Cu at (194.1, 118.9)
- added P1: USB_OTG, Connectors_USB:USB_Micro-B_Molex_47346-0001, F.Cu at (194.1, 62.5)
- added P1: USB_OTG, Connectors_USB:USB_Micro-B_Molex_47346-0001, F.Cu at (175.3, 81.3)
- added P1: USB_OTG, Connectors_USB:USB_Micro-B_Molex_47346-0001, F.Cu at (175.3, 100.1)
- added P1: USB_OTG, Connectors_USB:USB_Micro-B_Molex_47346-0001, F.Cu at (175.3, 118.9)
- added P1: USB_OTG, Connectors_USB:USB_Micro-B_Molex_47346-0001, F.Cu at (175.3, 62.5)
- added P1: USB_OTG, Connectors_USB:USB_Micro-B_Molex_47346-0001, F.Cu at (156.5, 81.3)
- added P2: LEFT, Pin_Headers:Pin_Header_Straight_1x06_Pitch2.54mm, B.Cu at (207.0, 110.1)
- added P2: LEFT, Pin_Headers:Pin_Header_Straight_1x06_Pitch2.54mm, B.Cu at (169.4, 91.3)
- added P2: LEFT, Pin_Headers:Pin_Header_Straight_1x06_Pitch2.54mm, B.Cu at (169.4, 53.7)
- added P2: LEFT, Pin_Headers:Pin_Header_Straight_1x06_Pitch2.54mm, B.Cu at (169.4, 72.5)
- added P2: LEFT, Pin_Headers:Pin_Header_Straight_1x06_Pitch2.54mm, B.Cu at (150.6, 110.1)
- added P2: LEFT, Pin_Headers:Pin_Header_Straight_1x06_Pitch2.54mm, B.Cu at (150.6, 91.3)
- added P2: LEFT, Pin_Headers:Pin_Header_Straight_1x06_Pitch2.54mm, B.Cu at (150.6, 53.7)
- added P2: LEFT, Pin_Headers:Pin_Header_Straight_1x06_Pitch2.54mm, B.Cu at (150.6, 72.5)
- added P2: LEFT, Pin_Headers:Pin_Header_Straight_1x06_Pitch2.54mm, B.Cu at (131.8, 91.3)
- added P2: LEFT, Pin_Headers:Pin_Header_Straight_1x06_Pitch2.54mm, B.Cu at (131.8, 110.1)
- added P2: LEFT, Pin_Headers:Pin_Header_Straight_1x06_Pitch2.54mm, B.Cu at (131.8, 72.5)
- added P2: LEFT, Pin_Headers:Pin_Header_Straight_1x06_Pitch2.54mm, B.Cu at (207.0, 91.3)
- added P2: LEFT, Pin_Headers:Pin_Header_Straight_1x06_Pitch2.54mm, B.Cu at (207.0, 53.7)
- added P2: LEFT, Pin_Headers:Pin_Header_Straight_1x06_Pitch2.54mm, B.Cu at (207.0, 72.5)
- added P2: LEFT, Pin_Headers:Pin_Header_Straight_1x06_Pitch2.54mm, B.Cu at (188.2, 110.1)
- added P2: LEFT, Pin_Headers:Pin_Header_Straight_1x06_Pitch2.54mm, B.Cu at (188.2, 91.3)
- added P2: LEFT, Pin_Headers:Pin_Header_Straight_1x06_Pitch2.54mm, B.Cu at (188.2, 53.7)
- added P2: LEFT, Pin_Headers:Pin_Header_Straight_1x06_Pitch2.54mm, B.Cu at (188.2, 72.5)
- added P2: LEFT, Pin_Headers:Pin_Header_Straight_1x06_Pitch2.54mm, B.Cu at (169.4, 110.1)
- added P3: RIGHT, Pin_Headers:Pin_Header_Straight_1x06_Pitch2.54mm, B.Cu at (207.0, 106.6)
- added P3: RIGHT, Pin_Headers:Pin_Header_Straight_1x06_Pitch2.54mm, B.Cu at (169.4, 125.3)
- added P3: RIGHT, Pin_Headers:Pin_Header_Straight_1x06_Pitch2.54mm, B.Cu at (169.4, 87.8)
- added P3: RIGHT, Pin_Headers:Pin_Header_Straight_1x06_Pitch2.54mm, B.Cu at (169.4, 69.0)
- added P3: RIGHT, Pin_Headers:Pin_Header_Straight_1x06_Pitch2.54mm, B.Cu at (150.6, 106.6)
- added P3: RIGHT, Pin_Headers:Pin_Header_Straight_1x06_Pitch2.54mm, B.Cu at (150.6, 125.3)
- added P3: RIGHT, Pin_Headers:Pin_Header_Straight_1x06_Pitch2.54mm, B.Cu at (150.6, 87.8)
- added P3: RIGHT, Pin_Headers:Pin_Header_Straight_1x06_Pitch2.54mm, B.Cu at (150.6, 69.0)
- added P3: RIGHT, Pin_Headers:Pin_Header_Straight_1x06_Pitch2.54mm, B.Cu at (131.8, 125.3)
- added P3: RIGHT, Pin_Headers:Pin_Header_Straight_1x06_Pitch2.54mm, B.Cu at (131.8, 106.6)
- added P3: RIGHT, Pin_Headers:Pin_Header_Straight_1x06_Pitch2.54mm, B.Cu at (131.8, 87.8)
- added P3: RIGHT, Pin_Headers:Pin_Header_Straight_1x06_Pitch2.54mm, B.Cu at (207.0, 125.3)
- added P3: RIGHT, Pin_Headers:Pin_Header_Straight_1x06_Pitch2.54mm, B.Cu at (207.0, 87.8)
- added P3: RIGHT, Pin_Headers:Pin_Header_Straight_1x06_Pitch2.54mm, B.Cu at (207.0, 69.0)
- added P3: RIGHT, Pin_Headers:Pin_Header_Straight_1x06_Pitch2.54mm, B.Cu at (188.2, 106.6)
- added P3: RIGHT, Pin_Headers:Pin_Header_Straight_1x06_Pitch2.54mm, B.Cu at (188.2, 125.3)
- added P3: RIGHT, Pin_Headers:Pin_Header_Straight_1x06_Pitch2.54mm, B.Cu at (188.2, 87.8)
- added P3: RIGHT, Pin_Headers:Pin_Header_Straight_1x06_Pitch2.54mm, B.Cu at (188.2, 69.0)
- added P3: RIGHT, Pin_Headers:Pin_Header_Straight_1x06_Pitch2.54mm, B.Cu at (169.4, 106.6)
- added R1: 22, Resistors_SMD:R_0603, F.Cu at (199.0, 78.6)
- added R1: 22, Resistors_SMD:R_0603, F.Cu at (161.4, 97.4)
- added R1: 22, Resistors_SMD:R_0603, F.Cu at (161.4, 116.2)
- added R1: 22, Resistors_SMD:R_0603, F.Cu at (161.4, 59.8)
- added R1: 22, Resistors_SMD:R_0603, F.Cu at (142.6, 78.6)
- added R1: 22, Resistors_SMD:R_0603, F.Cu at (142.6, 97.4)
- added R1: 22, Resistors_SMD:R_0603, F.Cu at (142.6, 116.2)
- added R1: 22, Resistors_SMD:R_0603, F.Cu at (142.6, 59.8)
- added R1: 22, Resistors_SMD:R_0603, F.Cu at (123.8, 116.2)
- added R1: 22, Resistors_SMD:R_0603, F.Cu at (123.8, 97.4)
- added R1: 22, Resistors_SMD:R_0603, F.Cu at (123.8, 78.6)
- added R1: 22, Resistors_SMD:R_0603, F.Cu at (199.0, 97.4)
- added R1: 22, Resistors_SMD:R_0603, F.Cu at (199.0, 116.2)
- added R1: 22, Resistors_SMD:R_0603, F.Cu at (199.0, 59.8)
- added R1: 22, Resistors_SMD:R_0603, F.Cu at (180.2, 78.6)
- added R1: 22, Resistors_SMD:R_0603, F.Cu at (180.2, 97.4)
- added R1: 22, Resistors_SMD:R_0603, F.Cu at (180.2, 116.2)
- added R1: 22, Resistors_SMD:R_0603, F.Cu at (180.2, 59.8)
- added R1: 22, Resistors_SMD:R_0603, F.Cu at (161.4, 78.6)
- added R2: 22, Resistors_SMD:R_0603, F.Cu at (199.0, 81.3)
- added R2: 22, Resistors_SMD:R_0603, F.Cu at (161.4, 100.1)
- added R2: 22, Resistors_SMD:R_0603, F.Cu at (161.4, 118.9)
- added R2: 22, Resistors_SMD:R_0603, F.Cu at (161.4, 62.5)
- added R2: 22, Resistors_SMD:R_0603, F.Cu at (142.6, 81.3)
- added R2: 22, Resistors_SMD:R_0603, F.Cu at (142.6, 100.1)
- added R2: 22, Resistors_SMD:R_0603, F.Cu at (142.6, 118.9)
- added R2: 22, Resistors_SMD:R_0603, F.Cu at (142.6, 62.5)
- added R2: 22, Resistors_SMD:R_0603, F.Cu at (123.8, 118.9)
- added R2: 22, Resistors_SMD:R_0603, F.Cu at (123.8, 100.1)
- added R2: 22, Resistors_SMD:R_0603, F.Cu at (123.8, 81.3)
- added R2: 22, Resistors_SMD:R_0603, F.Cu at (199.0, 100.1)
- added R2: 22, Resistors_SMD:R_0603, F.Cu at (199.0, 118.9)
- added R2: 22, Resistors_SMD:R_0603, F.Cu at (199.0, 62.5)
- added R2: 22, Resistors_SMD:R_0603, F.Cu at (180.2, 81.3)
- added R2: 22, Resistors_SMD:R_0603, F.Cu at (180.2, 100.1)
- added R2: 22, Resistors_SMD:R_0603, F.Cu at (180.2, 118.9)
- added R2: 22, Resistors_SMD:R_0603, F.Cu at (180.2, 62.5)
- added R2: 22, Resistors_SMD:R_0603, F.Cu at (161.4, 81.3)
- added R3: 330, Resistors_SMD:R_0603, F.Cu at (197.7, 94.5)
- added R3: 330, Resistors_SMD:R_0603, F.Cu at (160.1, 113.3)
- added R3: 330, Resistors_SMD:R_0603, F.Cu at (160.1, 75.7)
- added R3: 330, Resistors_SMD:R_0603, F.Cu at (160.1, 56.9)
- added R3: 330, Resistors_SMD:R_0603, F.Cu at (141.3, 94.5)
- added R3: 330, Resistors_SMD:R_0603, F.Cu at (141.3, 113.3)
- added R3: 330, Resistors_SMD:R_0603, F.Cu at (141.3, 75.7)
- added R3: 330, Resistors_SMD:R_0603, F.Cu at (141.3, 56.9)
- added R3: 330, Resistors_SMD:R_0603, F.Cu at (122.5, 113.3)
- added R3: 330, Resistors_SMD:R_0603, F.Cu at (122.5, 94.5)
- added R3: 330, Resistors_SMD:R_0603, F.Cu at (122.5, 75.7)
- added R3: 330, Resistors_SMD:R_0603, F.Cu at (197.7, 113.3)
- added R3: 330, Resistors_SMD:R_0603, F.Cu at (197.7, 75.7)
- added R3: 330, Resistors_SMD:R_0603, F.Cu at (197.7, 56.9)
- added R3: 330, Resistors_SMD:R_0603, F.Cu at (178.9, 94.5)
- added R3: 330, Resistors_SMD:R_0603, F.Cu at (178.9, 113.3)
- added R3: 330, Resistors_SMD:R_0603, F.Cu at (178.9, 75.7)
- added R3: 330, Resistors_SMD:R_0603, F.Cu at (178.9, 56.9)
- added R3: 330, Resistors_SMD:R_0603, F.Cu at (160.1, 94.5)
- added R4: 330, Resistors_SMD:R_0603, F.Cu at (207.8, 83.9)
- added R4: 330, Resistors_SMD:R_0603, F.Cu at (170.2, 102.7)
- added R4: 330, Resistors_SMD:R_0603, F.Cu at (170.2, 121.5)
- added R4: 330, Resistors_SMD:R_0603, F.Cu at (170.2, 65.2)
- added R4: 330, Resistors_SMD:R_0603, F.Cu at (151.4, 83.9)
- added R4: 330, Resistors_SMD:R_0603, F.Cu at (151.4, 102.7)
- added R4: 330, Resistors_SMD:R_0603, F.Cu at (151.4, 121.5)
- added R4: 330, Resistors_SMD:R_0603, F.Cu at (151.4, 65.2)
- added R4: 330, Resistors_SMD:R_0603, F.Cu at (132.6, 121.5)
- added R4: 330, Resistors_SMD:R_0603, F.Cu at (132.6, 102.7)
- added R4: 330, Resistors_SMD:R_0603, F.Cu at (132.6, 83.9)
- added R4: 330, Resistors_SMD:R_0603, F.Cu at (207.8, 102.7)
- added R4: 330, Resistors_SMD:R_0603, F.Cu at (207.8, 121.5)
- added R4: 330, Resistors_SMD:R_0603, F.Cu at (207.8, 65.2)
- added R4: 330, Resistors_SMD:R_0603, F.Cu at (189.0, 83.9)
- added R4: 330, Resistors_SMD:R_0603, F.Cu at (189.0, 102.7)
- added R4: 330, Resistors_SMD:R_0603, F.Cu at (189.0, 121.5)
- added R4: 330, Resistors_SMD:R_0603, F.Cu at (189.0, 65.2)
- added R4: 330, Resistors_SMD:R_0603, F.Cu at (170.2, 83.9)
- added R5: 330, Resistors_SMD:R_0603, F.Cu at (206.2, 83.9)
- added R5: 330, Resistors_SMD:R_0603, F.Cu at (168.7, 102.7)
- added R5: 330, Resistors_SMD:R_0603, F.Cu at (168.7, 121.5)
- added R5: 330, Resistors_SMD:R_0603, F.Cu at (168.7, 65.2)
- added R5: 330, Resistors_SMD:R_0603, F.Cu at (149.9, 83.9)
- added R5: 330, Resistors_SMD:R_0603, F.Cu at (149.9, 102.7)
- added R5: 330, Resistors_SMD:R_0603, F.Cu at (149.9, 121.5)
- added R5: 330, Resistors_SMD:R_0603, F.Cu at (149.9, 65.2)
- added R5: 330, Resistors_SMD:R_0603, F.Cu at (131.1, 121.5)
- added R5: 330, Resistors_SMD:R_0603, F.Cu at (131.1, 102.7)
- added R5: 330, Resistors_SMD:R_0603, F.Cu at (131.1, 83.9)
- added R5: 330, Resistors_SMD:R_0603, F.Cu at (206.2, 102.7)
- added R5: 330, Resistors_SMD:R_0603, F.Cu at (206.2, 121.5)
- added R5: 330, Resistors_SMD:R_0603, F.Cu at (206.2, 65.2)
- added R5: 330, Resistors_SMD:R_0603, F.Cu at (187.5, 83.9)
- added R5: 330, Resistors_SMD:R_0603, F.Cu at (187.5, 102.7)
- added R5: 330, Resistors_SMD:R_0603, F.Cu at (187.5, 121.5)
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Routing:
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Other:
- board size 81.8 x 90.9 mm -> 91.4 x 85.3 mm
- board text added: "HASL Pb FREE 1.6mm FR4 RED SOLDERMASK THUNKIT ELECTRONICS"
